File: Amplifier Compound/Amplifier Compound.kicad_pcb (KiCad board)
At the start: 2 copper layers, 77.7 x 60 mm, 52 parts, among them J1 Screw_Terminal_01x02, J3 Screw_Terminal_01x02, U1 PA88, U2 LT1012

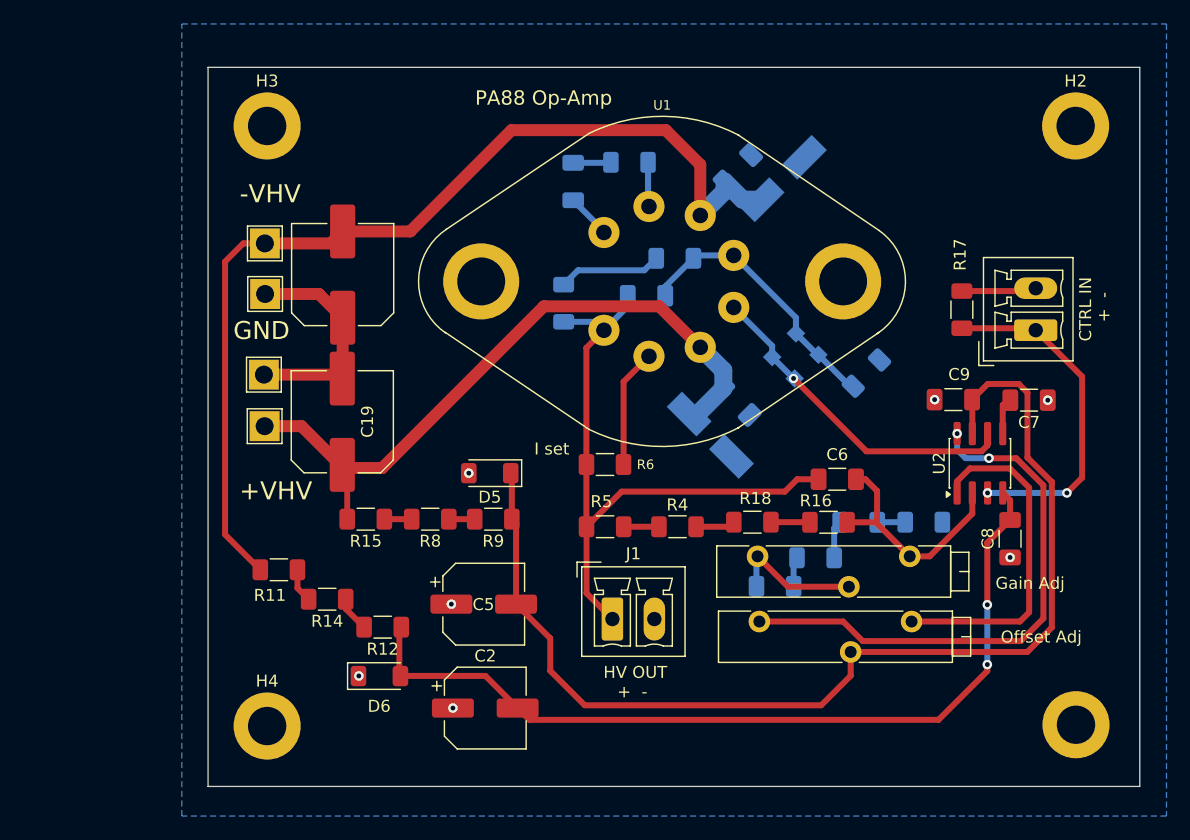
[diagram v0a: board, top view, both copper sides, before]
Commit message: update composite
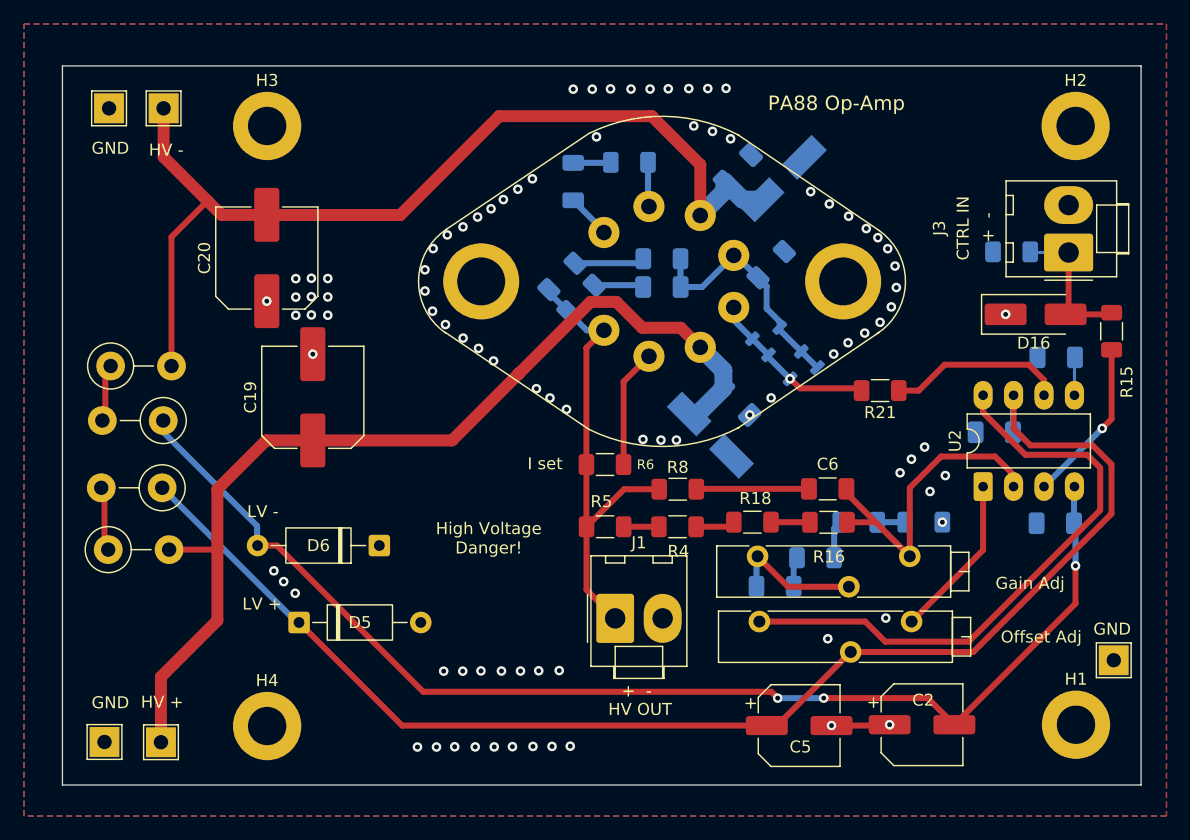
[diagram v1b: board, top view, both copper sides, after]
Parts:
- removed D1, D2: DSS120U, Diode_SMD:D_SOD-123F
- added D16: SMA6J12CA, Diode_SMD:D_SMA_Handsoldering, F.Cu at (199.7, 82.7)
- added Q1: MMBF5457, Package_TO_SOT_SMD:SOT-23-3, B.Cu at (180.1, 87.2)
- added Q2: MMBF5457, Package_TO_SOT_SMD:SOT-23-3, B.Cu at (177.6, 84.6)
- added R21: 10k, Resistor_SMD:R_1206_3216Metric_Pad1.30x1.75mm_HandSolder, F.Cu at (186.8, 89.0)
- added R22: 220k, Resistor_THT:R_Axial_DIN0411_L9.9mm_D3.6mm_P5.08mm_Vertical, F.Cu at (122.6, 87.0)
- added TP5: GND, TestPoint:TestPoint_THTPad_2.5x2.5mm_Drill1.2mm, F.Cu at (206.3, 111.5)
- C10, C6: value 15pF -> 6.6pF
- C2, C5: value 200pf -> 100uf
- C7, C8, C9: moved to B.Cu
- D5, D6: value D_Zener 15V -> D_Zener 18V; footprint Diode_SMD:D_MiniMELF -> Diode_THT:D_A-405_P10.16mm_Horizontal
- H1, H2, H3, H4: footprint MountingHole:MountingHole_3.2mm_M3_DIN965_Pad -> MountingHole:MountingHole_3.2mm_M3_ISO7380_Pad
- J1, J3: footprint Connector_Phoenix_MC:PhoenixContact_MCV_1,5_2-G-3.5_1x02_P3.50mm_Vertical -> Connector_Molex:Molex_KK-396_A-41791-0002_1x02_P3.96mm_Vertical
- R11, R12, R14: value 68k -> 220k; footprint Resistor_SMD:R_1206_3216Metric_Pad1.30x1.75mm_HandSolder -> Resistor_THT:R_Axial_DIN0411_L9.9mm_D3.6mm_P5.08mm_Vertical
- R15: value 68k -> 10k
- R17: value NC -> 10M; moved to B.Cu
- R8: value 68k -> 100R
- R9: value 68K -> 100R; moved to B.Cu
- U2: footprint Package_SO:SOIC-8_3.9x4.9mm_P1.27mm -> Package_DIP:DIP-8_W7.62mm_LongPads
- moved R15 64.2 mm to (206.1, 84.1), turned to 90 degrees
- moved C2 36.5 mm to (190.3, 116.9)
- moved TP4 33.4 mm to (122.0, 118.3), turned to 180 degrees
- moved C5 28.2 mm to (180.0, 117.0)
- moved TP1 27.8 mm to (126.8, 118.4), turned to 180 degrees
- moved R12 23.8 mm to (122.4, 102.3), turned to 0 degrees
- moved R8 20.8 mm to (169.9, 97.2), turned to 0 degrees
- moved TP3 20.2 mm to (122.4, 65.5), turned to -90 degrees
- moved D5 20.2 mm to (138.3, 108.4), turned to 0 degrees
- moved R9 19.8 mm to (161.8, 81.3), turned to 45 degrees
- moved R14 16.6 mm to (126.9, 97.1)
- moved R11 15.8 mm to (127.0, 91.5)
- moved TP2 14.1 mm to (127.0, 65.5), turned to -90 degrees
- moved R13 12.0 mm to (177.7, 78.5)
- moved D6 10.9 mm to (145.0, 102.0), turned to 180 degrees
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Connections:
- C10 pad 2: /HVOUT -> Net-(C10-Pad2)
- C5 pad 1: GND -> +VLV
- C5 pad 2: +VLV -> GND
- C6 pad 2: /HVOUT -> Net-(C6-Pad2)
- H2 pad 1: unconnected-(H2-Pad1) -> GND
- H4 pad 1: unconnected-(H4-Pad1) -> GND
- J3 pad 1: Net-(J3-Pin_1) -> Net-(D16-A2)
- R11 pad 1: Net-(R11-Pad1) -> -VLV
- R11 pad 2: -VHV -> Net-(R11-Pad2)
- R12 pad 1: -VLV -> Net-(R12-Pad1)
- R12 pad 2: Net-(R12-Pad2) -> +VHV
- R14 pad 1: Net-(R12-Pad2) -> +VLV
- R14 pad 2: Net-(R11-Pad1) -> Net-(R12-Pad1)
- R15 pad 1: Net-(R15-Pad1) -> Net-(U2-+)
- R15 pad 2: +VHV -> Net-(D16-A2)
- R17 pad 1: Net-(J3-Pin_1) -> GND
- R17 pad 2: GND -> Net-(D16-A2)
- R8 pad 1: Net-(R8-Pad1) -> /HVOUT
- R8 pad 2: Net-(R15-Pad1) -> Net-(C6-Pad2)
- R9 pad 1: +VLV -> /HVOUT
- R9 pad 2: Net-(R8-Pad1) -> Net-(C10-Pad2)
- U1 pad 4: /CTRL -> Net-(Q1-G)
- U2 pad 3: Net-(J3-Pin_1) -> Net-(U2-+)
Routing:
- net Net-(J3-Pin_1): track 29.1 -> 0.00 mm, vias 2 -> 0
- net -VLV: track 72.8 -> 101.9 mm, vias 2 -> 3
- net +VHV: track 57.2 -> 83.5 mm
- net GND: track 27.1 -> 2.73 mm, vias 7 -> 90
- net +VLV: track 93.8 -> 113.2 mm
- net Net-(U2-BAL): track 28.6 -> 13.7 mm
- net /HVOUT: track 54.0 -> 39.2 mm
- net Net-(Q1-G): track 0.00 -> 14.3 mm, vias 0 -> 1
- net Net-(U2-+): track 0.00 -> 13.7 mm, vias 0 -> 1
- net /CTRL: track 27.9 -> 14.8 mm, vias 1 -> 0
- net Net-(D16-A2): track 0.00 -> 12.4 mm
- net Net-(C6-Pad2): track 0.00 -> 9.41 mm
- net Net-(U2--): track 20.2 -> 27.3 mm
- net Net-(R11-Pad2): track 0.00 -> 4.84 mm
- net Net-(R12-Pad1): track 0.00 -> 4.80 mm
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- added copper zone on F.Cu, net GND
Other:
- board size 77.7 x 60 mm -> 90 x 60 mm
- board text added: "HV +"
- board text added: "HV -"
- board text added: "High Voltage Danger!"
- board text added: "LV +"
- board text added: "LV -"
- board text removed: "+VHV"
- board text removed: "-VHV"
